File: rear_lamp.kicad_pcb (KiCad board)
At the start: 2 copper layers, 14 parts, among them J1 PWR, Q1 BD138, Q2 BC856, Q3 BC847

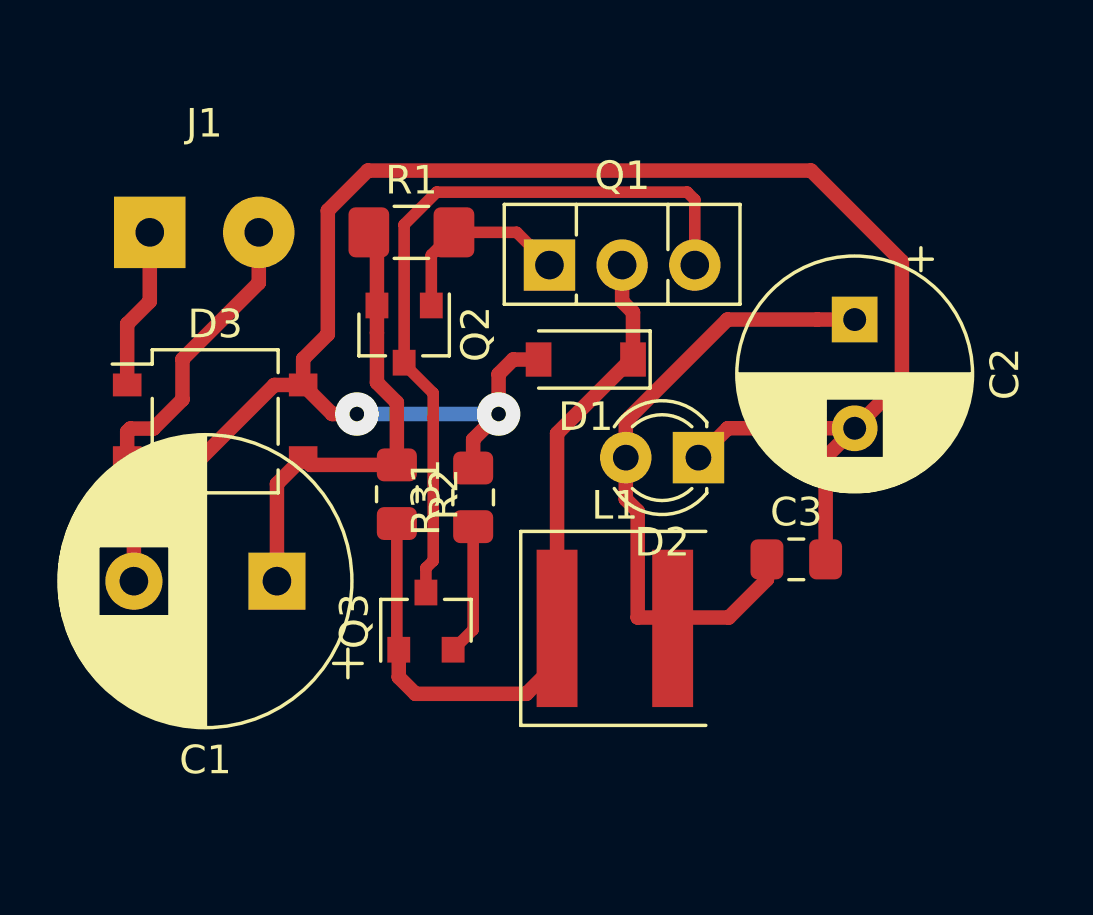
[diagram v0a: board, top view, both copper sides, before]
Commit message: one plane
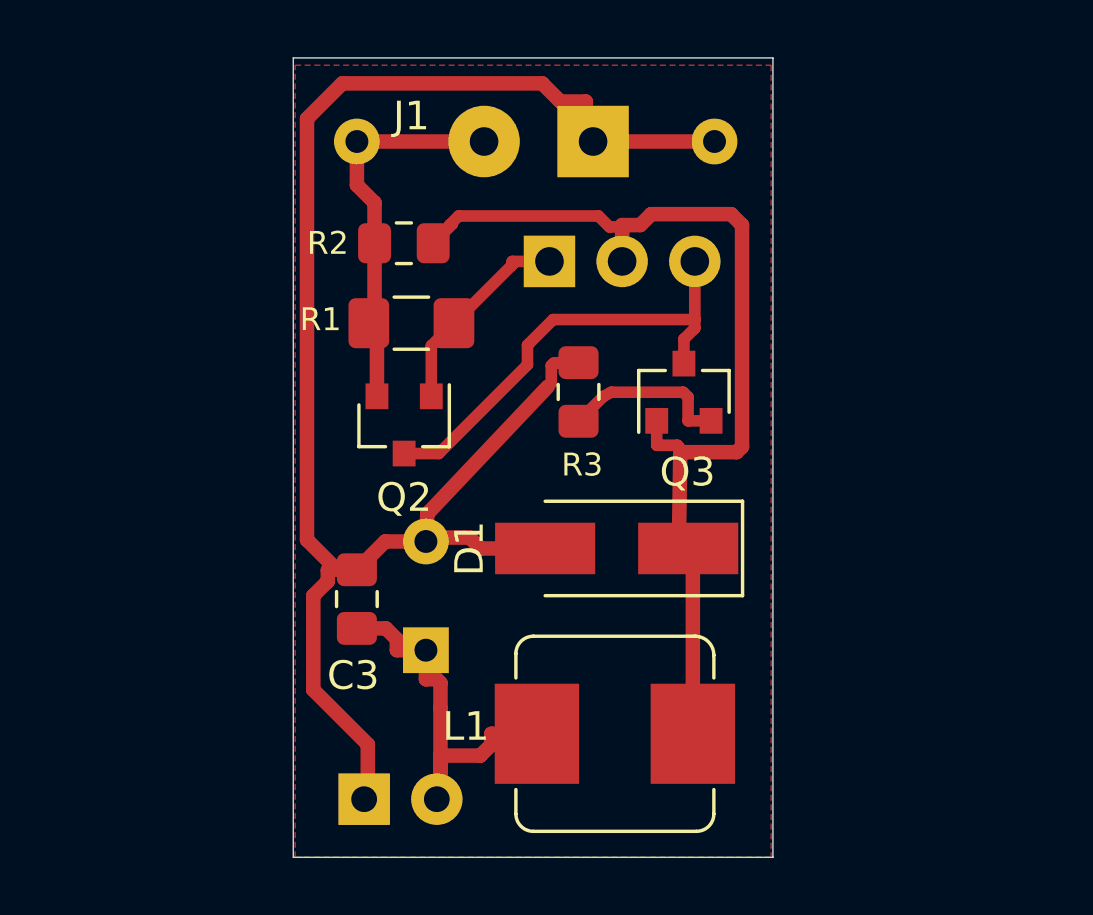
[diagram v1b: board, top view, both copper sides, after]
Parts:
- removed D3: MB6S, Package_TO_SOT_SMD:TO-269AA
- C1: footprint Capacitor_THT:CP_Radial_D10.0mm_P5.00mm -> Capacitor_THT:C_Axial_L5.1mm_D3.1mm_P12.50mm_Horizontal; moved to B.Cu
- C2, Q1: moved to B.Cu
- D1: footprint Diode_SMD:D_SOD-123 -> Diode_SMD:D_SMA_Handsoldering
- D2: footprint LED_THT:LED_D3.0mm -> LED_THT:LED_D4.0mm; moved to B.Cu
- L1: footprint Inductor_SMD:L_Coilcraft_XAL60xx_6.36x6.56mm -> Inductor_SMD:L_Bourns_SRP7028A_7.3x6.6mm
- moved C2 18.9 mm to (46.2, 42.4), turned to 90 degrees
- moved D2 16.7 mm to (44.1, 47.6), turned to 0 degrees
- moved J1 15.8 mm to (52.1, 24.6), turned to 180 degrees
- moved C1 15.6 mm to (43.8, 24.6), turned to 0 degrees
- moved C3 15.4 mm to (43.8, 40.6), turned to 90 degrees
- moved Q3 12.1 mm to (55.2, 33.4)
- moved R2 8.78 mm to (45.5, 28.2), turned to 0 degrees
- moved D1 6.69 mm to (52.9, 38.9)
- moved R3 5.21 mm to (51.6, 33.4)
- moved L1 3.68 mm to (52.8, 45.3), turned to 180 degrees
- moved R1 3.18 mm to (45.7, 31.0)
- moved Q2 3.17 mm to (45.5, 34.5)
- moved Q1 0.13 mm to (50.5, 28.8)
- renumbered R31 to R3
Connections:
- J1 pad 1: Net-(D3-Pad1) -> GND
- J1 pad 2: Net-(D3-Pad2) -> VCC
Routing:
- net Net-(D3-Pad2): track 10.3 -> 0.00 mm
- net Net-(Q1-Pad3): track 26.4 -> 16.2 mm
- net GND: track 68.2 -> 58.7 mm, vias 2 -> 0
- net Net-(C2-Pad1): track 22.5 -> 13.0 mm
- net Net-(D1-Pad1): track 26.8 -> 33.8 mm
- net Net-(D3-Pad1): track 5.66 -> 0.00 mm
- net VCC: track 16.6 -> 13.8 mm
- net Net-(Q3-Pad2): track 4.59 -> 5.93 mm
- added copper zone on F.Cu, net GND
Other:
- board outline added: 16.8 x 27.9 mm
- net class PWR removed
- net class pwr added: clearance 0.2, trace_width 0.508, via_dia 0.8, via_drill 0.4
- net class signal added: clearance 0.2, trace_width 0.4064, via_dia 0.8, via_drill 0.4

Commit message: small pcb
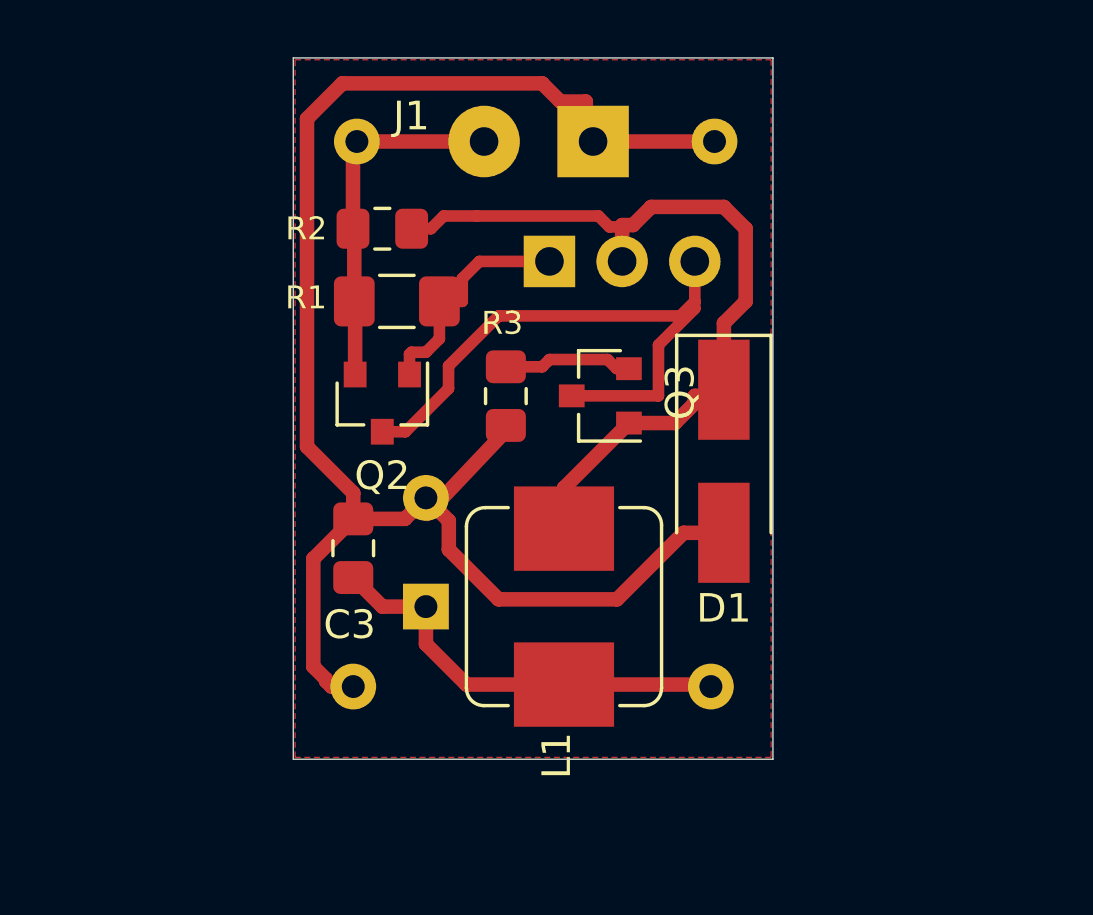
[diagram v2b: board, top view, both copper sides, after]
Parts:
- D2: footprint LED_THT:LED_D4.0mm -> Capacitor_THT:C_Axial_L5.1mm_D3.1mm_P12.50mm_Horizontal
- moved D1 4.83 mm to (56.6, 35.8), turned to 270 degrees
- moved L1 4.79 mm to (51.1, 40.9), turned to 270 degrees
- moved D2 3.96 mm to (43.7, 43.7)
- moved Q3 2.92 mm to (52.3, 33.5), turned to 180 degrees
- moved R3 2.54 mm to (49.0, 33.5), turned to 270 degrees
- moved C3 1.78 mm to (43.7, 38.9)
- moved C2 1.52 mm to (46.2, 40.9)
- moved Q2 1.08 mm to (44.7, 33.8)
- moved R1 0.92 mm to (45.2, 30.2)
- moved R2 0.91 mm to (44.7, 27.7)
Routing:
- net Net-(D1-Pad1): track 33.8 -> 28.5 mm
- net Net-(Q1-Pad3): track 16.2 -> 21.5 mm
- net Net-(C2-Pad1): track 13.0 -> 14.8 mm
- net Net-(Q3-Pad2): track 5.93 -> 4.54 mm
- net VCC: track 13.8 -> 12.7 mm
- net Net-(Q1-Pad1): track 7.19 -> 8.18 mm
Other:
- board size 16.8 x 27.9 mm -> 16.8 x 24.5 mm
